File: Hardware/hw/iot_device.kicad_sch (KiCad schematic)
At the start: 36 parts, among them J3 Conn_01x04_Pin, J4 USB4085-GF-A_REVA4, Q6 PMOS, Q7 PMOS, SW1 SW_Push, SW2 SW_Push, U4 ESP32-C6-WROOM-1, U5 TPS63001, U6 USBLC6-4SC6, U7 RV-3028-C7

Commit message: Stupid-Stupid update
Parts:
- L1: footprint Inductor_SMD:L_6.3x6.3_H3 -> Inductor_SMD:L_Taiyo-Yuden_NR-60xx
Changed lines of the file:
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@@
 			)
 		)
-		(property "Footprint" "Inductor_SMD:L_6.3x6.3_H3"
+		(property "Footprint" "Inductor_SMD:L_Taiyo-Yuden_NR-60xx"
 			(at 77.47 172.72 0)
 			(effects

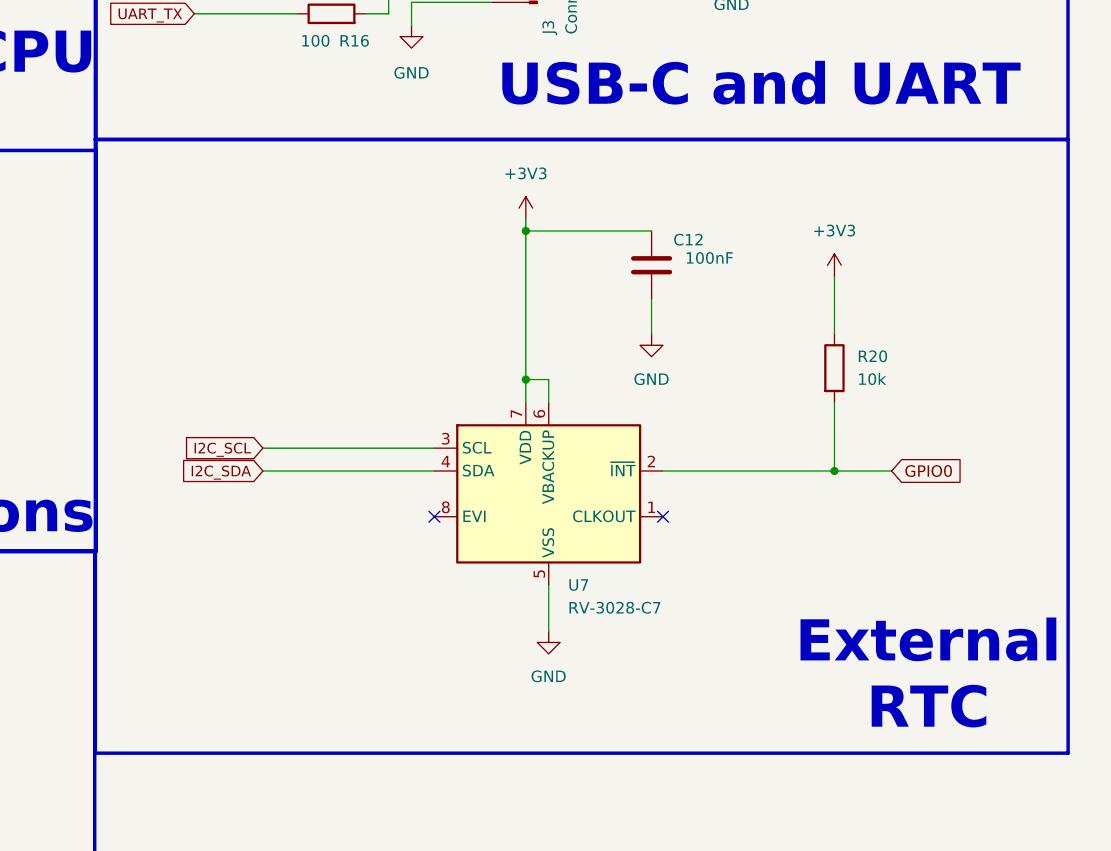
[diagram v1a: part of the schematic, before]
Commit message: RTC update
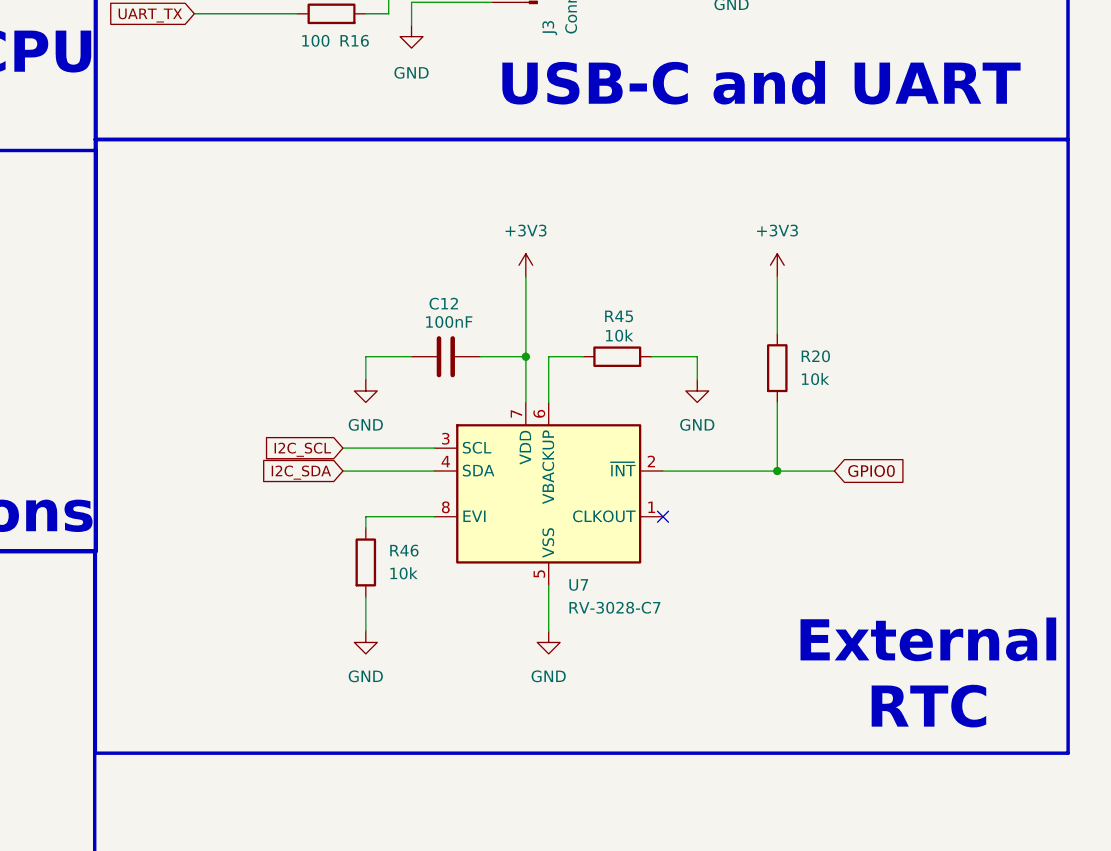
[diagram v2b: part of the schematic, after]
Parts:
- added R45, R46: 10k, Resistor_SMD:R_0805_2012Metric, symbol Device:R
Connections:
- net +3V3: no longer U7.6 (VBACKUP)
- net GND: now also R45.2, R46.2
- net at U7.8 (EVI): now also R46.1
- new net: R45.1, U7.6 (VBACKUP)
- no-connect marks 9 -> 8
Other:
- moved on the sheet: C12, R20
